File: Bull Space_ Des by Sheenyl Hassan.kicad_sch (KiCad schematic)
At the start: 24 parts, among them IC1 TEENSY_4.0, IC2 XB24CZ7PIT-004, J1 Screw_Terminal_01x06, Q4 2N7002, U1 VXO7803-1000, U2 Flight-Computer_Adafruit_GPS_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, U3 ADXL345, U4 BMP280, U6 Memory_Flash_W25Q32JVSS

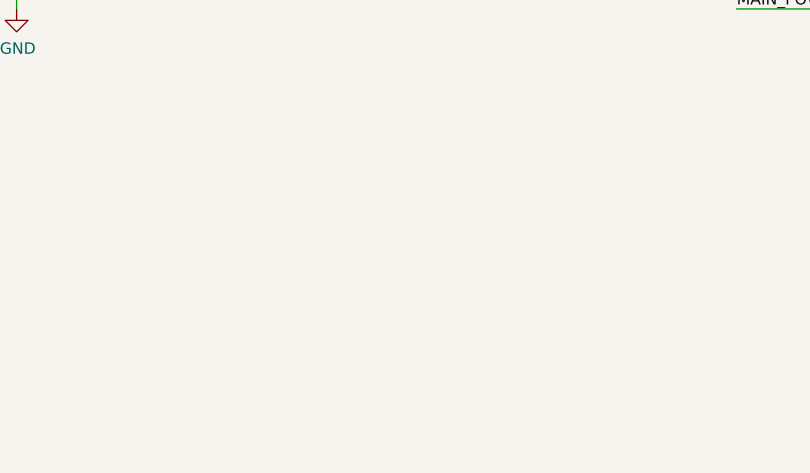
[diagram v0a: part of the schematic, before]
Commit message: Added UB SEDS Logo
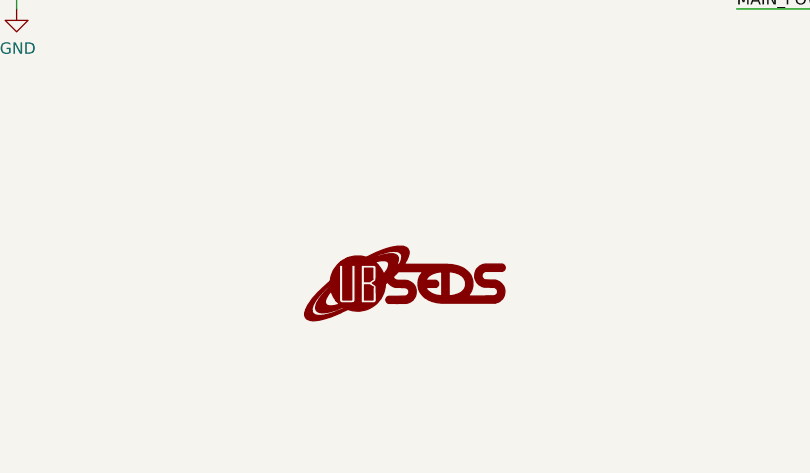
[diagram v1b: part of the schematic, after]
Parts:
- added G1: UB-SEDS-Logo, Flight Computer:SEDS_logo_soldermask, symbol Flight-Computer:UB-SEDS-Logo
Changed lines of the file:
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@@
     (pin "1")
+  )
+  (symbol (lib_id "Flight-Computer:UB-SEDS-Logo") (at 193.04 173.99 0) (unit 1)
+    (in_bom yes) (on_board yes) (fields_autoplaced)
+    (property "Reference" "G1" (id 0) (at 193.04 177.4698 0)
+      (effects (font (size 1.524 1.524)) hide)
+    )
+    (property "Value" "UB-SEDS-Logo" (id 1) (at 193.04 170.5102 0)
+      (effects (font (size 1.524 1.524)) hide)
+    )
+    (property "Footprint" "Flight Computer:SEDS_logo_soldermask" (id 2) (at 193.04 173.99 0)
+      (effects (font (size 1.524 1.524)) hide)
+    )
+    (property "Datasheet" "" (id 3) (at 193.04 173.99 0)
+      (effects (font (size 1.524 1.524)) hide)
+    )
   )
   (symbol (lib_id "Device:R") (at 238.76 81.28 270) (unit 1)
@@
       (reference "F2") (unit 1) (value "3A Polyfuse") (footprint "Fuse:Fuse_1206_3216Metric_Pad1.42x1.75mm_HandSolder")
     )
+    (path "/62a0b005-d543-412f-93b9-72a8d1c3610c"
+      (reference "G1") (unit 1) (value "UB-SEDS-Logo") (footprint "Flight Computer:SEDS_logo_soldermask")
+    )
     (path "/098fe236-6563-41cf-9ea3-cdb345516ea9"

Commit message: Add files via upload
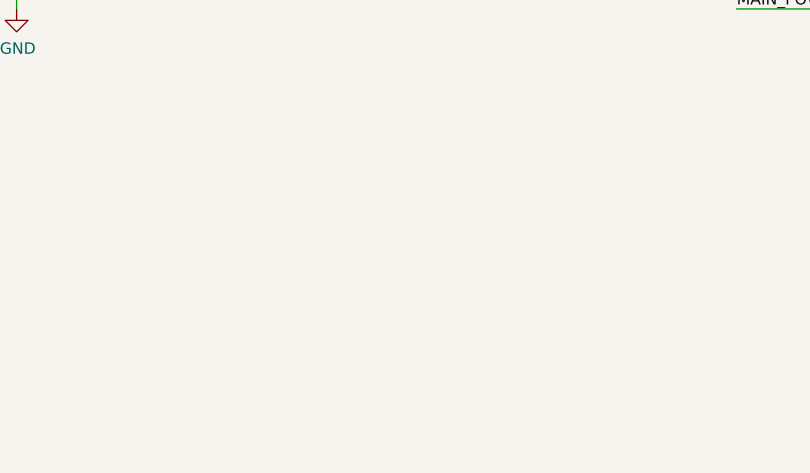
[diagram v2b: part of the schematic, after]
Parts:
- removed G1: UB-SEDS-Logo, Flight Computer:SEDS_logo_soldermask, symbol Flight-Computer:UB-SEDS-Logo
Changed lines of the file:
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@@
     (pin "1")
-  )
-  (symbol (lib_id "Flight-Computer:UB-SEDS-Logo") (at 193.04 173.99 0) (unit 1)
-    (in_bom yes) (on_board yes) (fields_autoplaced)
-    (property "Reference" "G1" (id 0) (at 193.04 177.4698 0)
-      (effects (font (size 1.524 1.524)) hide)
-    )
-    (property "Value" "UB-SEDS-Logo" (id 1) (at 193.04 170.5102 0)
-      (effects (font (size 1.524 1.524)) hide)
-    )
-    (property "Footprint" "Flight Computer:SEDS_logo_soldermask" (id 2) (at 193.04 173.99 0)
-      (effects (font (size 1.524 1.524)) hide)
-    )
-    (property "Datasheet" "" (id 3) (at 193.04 173.99 0)
-      (effects (font (size 1.524 1.524)) hide)
-    )
   )
   (symbol (lib_id "Device:R") (at 238.76 81.28 270) (unit 1)
@@
       (reference "F2") (unit 1) (value "3A Polyfuse") (footprint "Fuse:Fuse_1206_3216Metric_Pad1.42x1.75mm_HandSolder")
     )
-    (path "/62a0b005-d543-412f-93b9-72a8d1c3610c"
-      (reference "G1") (unit 1) (value "UB-SEDS-Logo") (footprint "Flight Computer:SEDS_logo_soldermask")
-    )
     (path "/098fe236-6563-41cf-9ea3-cdb345516ea9"
